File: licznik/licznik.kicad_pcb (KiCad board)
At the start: 2 copper layers, 72 x 44.1 mm, 66 parts, among them J4 1140084168, J5 Conn_01x03_Female, U1 AMS1117-3.3, U2 AMS1117-5.0, U6 oled, Y1 Crystal

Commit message: wip
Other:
- net class Default removed

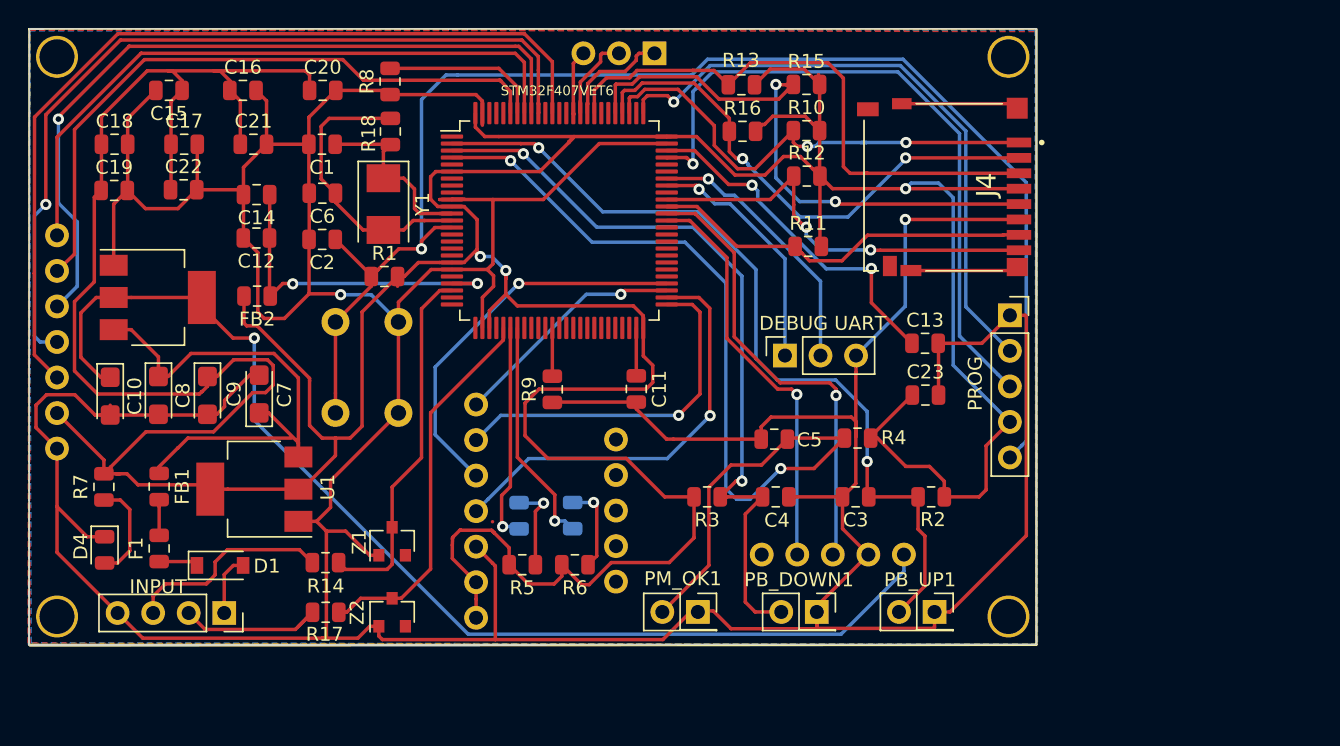
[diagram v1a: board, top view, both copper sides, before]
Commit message: hardware_2
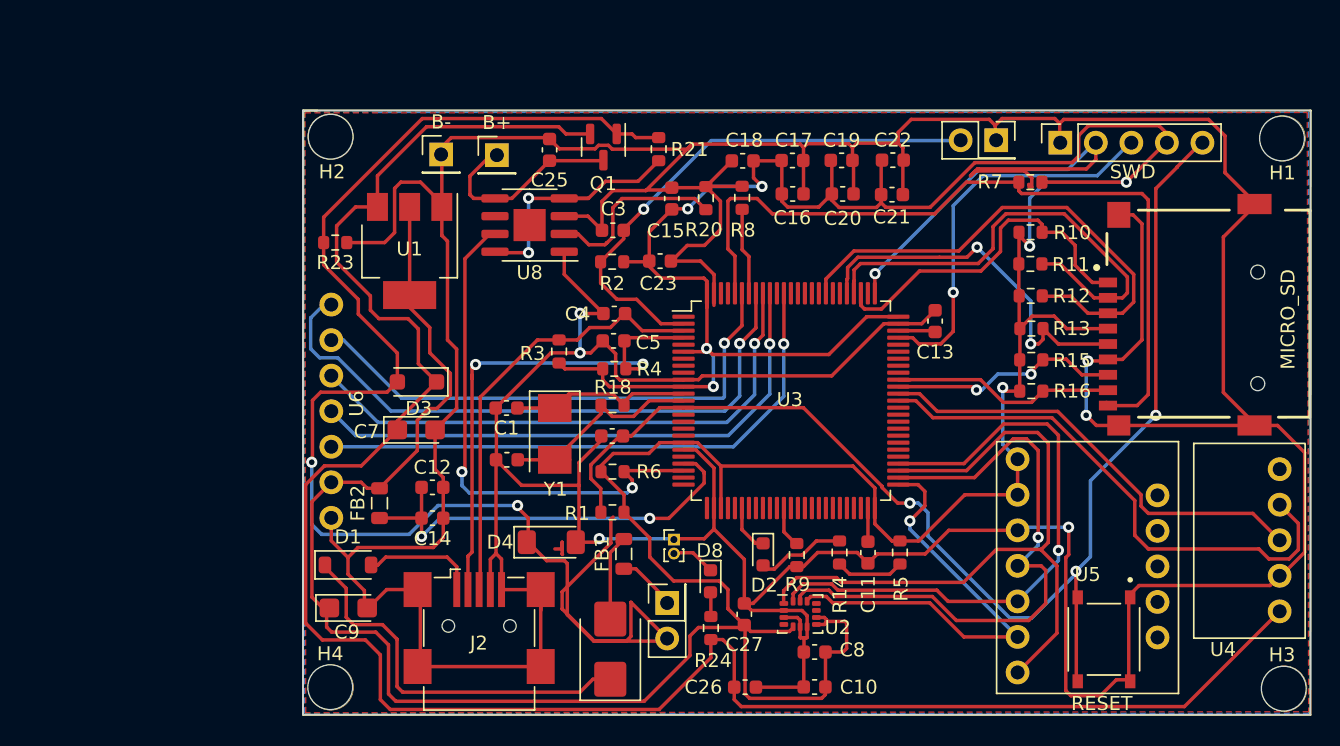
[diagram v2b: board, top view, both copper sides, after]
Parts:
- removed  LSM6DS3: gyro, licznik:gy1
- removed DEBUG UART: Conn_01x03_Female, Connector_PinSocket_2.54mm:PinSocket_1x03_P2.54mm_Vertical
- removed GPS NEO-6M: gps, licznik:gp1
- removed INPUT: Conn_01x04_Female, Connector_PinSocket_2.54mm:PinSocket_1x04_P2.54mm_Vertical
- removed J4: 1140084168, licznik:AMPHENOL_1140084168
- removed J5: Conn_01x03_Female, Connector_PinSocket_2.54mm:PinSocket_1x03_P2.54mm_Vertical
- removed PB_DOWN1, PB_UP1: SW_Push, Connector_PinSocket_2.54mm:PinSocket_2x01_P2.54mm_Vertical
- removed PM_OK1: PB_OK, Connector_PinSocket_2.54mm:PinSocket_2x01_P2.54mm_Vertical
- removed PROG: Conn_01x05_Female, Connector_PinSocket_2.54mm:PinSocket_1x05_P2.54mm_Vertical
- removed R17: 510R, Resistor_SMD:R_0805_2012Metric
- removed RESET1: SW_Push, Button_Switch_THT:SW_PUSH_6mm
- removed STM32F407VET6: STM32F407VETx, Package_QFP:LQFP-100_14x14mm_P0.5mm
- removed Z1, Z2: KDZ3.3V-RTK/P, Diode_SMD:D_SOT-23_ANK
- added B+: BAT+, Connector_PinHeader_2.54mm:PinHeader_1x01_P2.54mm_Vertical, F.Cu at (123.1, 71.7)
- added B-: BAT-, Connector_PinHeader_2.54mm:PinHeader_1x01_P2.54mm_Vertical, F.Cu at (119.1, 71.6)
- added C25: 10uF, Capacitor_SMD:C_0603_1608Metric, F.Cu at (126.8, 71.3)
- added C26: 22uF, Capacitor_SMD:C_0603_1608Metric, F.Cu at (140.8, 109.7)
- added C27: 22uF, Capacitor_SMD:C_0603_1608Metric, F.Cu at (140.8, 104.5)
- added D8: LED, LED_SMD:LED_0603_1608Metric, F.Cu at (138.4, 102.1)
- added H1: MountingHole_Pad, MountingHole:MountingHole_3.2mm_M3, F.Cu at (179.2, 70.5)
- added H2: MountingHole_Pad, MountingHole:MountingHole_3.2mm_M3, F.Cu at (111.2, 70.4)
- added H3: MountingHole_Pad, MountingHole:MountingHole_3.2mm_M3, F.Cu at (179.3, 109.8)
- added H4: MountingHole_Pad, MountingHole:MountingHole_3.2mm_M3, F.Cu at (111.2, 109.7)
- added J2: USB_B_Mini, Connector_USB:USB_Mini-B_Wuerth_65100516121_Horizontal, F.Cu at (121.8, 105.3)
- added LEN_ON: jump, Connector_PinHeader_1.00mm:PinHeader_1x02_P1.00mm_Vertical, F.Cu at (135.7, 99.2)
- added MICRO_SD: TF-01A, slot_sd:TF-01A, F.Cu at (173.9, 83.0)
- added PB_POWER: POWER_PB, Connector_PinSocket_2.54mm:PinSocket_2x01_P2.54mm_Vertical, F.Cu at (135.3, 103.7)
- added PB_UP: SW_Push, Connector_PinSocket_2.54mm:PinSocket_2x01_P2.54mm_Vertical, F.Cu at (158.8, 70.6)
- added Q1: AO3401A, Package_TO_SOT_SMD:SOT-23, F.Cu at (130.7, 71.1)
- added R20: 2K, Resistor_SMD:R_0603_1608Metric, F.Cu at (138.0, 74.8)
- added R21: 0.1R, Resistor_SMD:R_0603_1608Metric, F.Cu at (134.7, 71.2)
- added R23: 10K, Resistor_SMD:R_0603_1608Metric, F.Cu at (111.5, 77.9)
- added R24: 2K, Resistor_SMD:R_0603_1608Metric, F.Cu at (138.4, 105.5)
- added RESET: USER_PB, TS_1187A-B-A-B:SW_TS-1187A-B-A-B, F.Cu at (166.5, 106.3)
- added SWD: Conn_01x05_Female, Connector_PinSocket_2.54mm:PinSocket_1x05_P2.54mm_Vertical, F.Cu at (163.4, 70.8)
- added U3: STM32F407VETx, Package_QFP:LQFP-100_14x14mm_P0.5mm, F.Cu at (144.1, 89.2)
- added U4: gps, licznik:gp1, F.Cu at (176.7, 99.7)
- added U5: gyro, licznik:gy1, F.Cu at (165.3, 101.2)
- added U8: TP4056, Package_SO:HSOP-8-1EP_3.9x4.9mm_P1.27mm_EP2.3x2.3mm, F.Cu at (125.4, 76.7)
- C1, C11, C12, C13, C14, C15, C16, C17, C18, C19, C2, C20, C21, C22, C23, C3, C4, C5, C6: footprint Capacitor_SMD:C_0805_2012Metric -> Capacitor_SMD:C_0603_1608Metric
- C10, C8: value 10uF -> 100nF; footprint Capacitor_Tantalum_SMD:CP_EIA-3216-18_Kemet-A -> Capacitor_SMD:C_0603_1608Metric
- D2: footprint LED_SMD:LED_0805_2012Metric -> LED_SMD:LED_0603_1608Metric; moved to F.Cu
- D3: value LED -> SM4007; footprint LED_SMD:LED_0805_2012Metric -> Diode_SMD:D_SOD-123F; moved to F.Cu
- D4: value LED -> ZMMxx; footprint LED_SMD:LED_0805_2012Metric -> Diode_SMD:D_MiniMELF
- F1: footprint Fuse:Fuse_0805_2012Metric -> Diode_SMD:D_SMB
- R1, R10, R11, R12, R13, R15, R16, R18, R2, R3, R4, R5, R8, R9: footprint Resistor_SMD:R_0805_2012Metric -> Resistor_SMD:R_0603_1608Metric
- R14: value 510R -> 0R; footprint Resistor_SMD:R_0805_2012Metric -> Resistor_SMD:R_0603_1608Metric
- R6, R7: value 510R -> 10K; footprint Resistor_SMD:R_0805_2012Metric -> Resistor_SMD:R_0603_1608Metric
- U2: value AMS1117-5.0 -> LSM6DS3; footprint Package_TO_SOT_SMD:SOT-223-3_TabPin2 -> Package_LGA:LGA-14_3x2.5mm_P0.5mm_LayoutBorder3x4y
- moved R7 69.7 mm to (161.2, 73.6), turned to 0 degrees
- moved C10 54.5 mm to (145.8, 109.7), turned to 0 degrees
- moved C19 52.0 mm to (147.7, 72.0)
- moved U2 51.2 mm to (144.8, 104.5)
- moved C22 50.7 mm to (151.4, 72.0)
- moved C8 50.4 mm to (145.8, 107.2), turned to 180 degrees
- moved C21 45.8 mm to (151.3, 74.5)
- moved C18 44.9 mm to (140.7, 72.1), turned to 180 degrees
- moved C17 43.5 mm to (144.2, 72.1)
- moved C16 40.0 mm to (144.2, 74.5)
- moved C20 37.9 mm to (147.8, 74.5)
- moved C15 36.8 mm to (135.6, 74.8), turned to 90 degrees
- moved R14 36.7 mm to (147.6, 100.1), turned to -90 degrees
- moved FB1 33.6 mm to (132.2, 100.2), turned to 90 degrees
- moved F1 33.0 mm to (131.2, 107.0)
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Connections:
- C10 pad 1: +5V -> GND
- C10 pad 2: GND -> +3V3
- C7 pad 1: Net-(C7-Pad1) -> REG_IN
- C8 pad 1: Net-(C7-Pad1) -> +3V3
- D1 pad 2: +12V -> Net-(D1-A)
- D2 pad 2: Net-(D2-Pad2) -> Net-(D2-A)
- D3 pad 1: LED_2 -> REG_IN
- D3 pad 2: Net-(D3-Pad2) -> +5V
- D4 pad 1: GND -> +5V
- D4 pad 2: Net-(D4-Pad2) -> GND
- FB1 pad 1: Net-(C7-Pad1) -> Net-(FB1-Pad1)
- R11 pad 1: SDIO_D0 -> SDIO_D3
- R12 pad 1: SDIO_D1 -> SDIO_CMD
- R13 pad 1: SDIO_CMD -> SDIO_SCK
- R14 pad 1: Net-(J3-Pad3) -> Net-(D2-A)
- R14 pad 2: ENGINE_RPM_INPUT -> Net-(R14-Pad2)
- R15 pad 1: SDIO_SCK -> SDIO_D0
- R16 pad 1: SDIO_D3 -> SDIO_D1
- R5 pad 1: Net-(D2-Pad2) -> Net-(R14-Pad2)
- R6 pad 1: Net-(D3-Pad2) -> CHRG_SIGNAL
- R7 pad 1: Net-(D4-Pad2) -> SDIO_INSERT_CARD
- U1 pad 3: Net-(C7-Pad1) -> REG_IN
- U2 pad 1: GND -> GYRO_MISO
- U2 pad 2: +5V -> GND
- U2 pad 3: Net-(C7-Pad1) -> GND
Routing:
- net REG_IN: track 0.00 -> 145.0 mm
- net GND: track 373.0 -> 443.6 mm, vias 2 -> 6
- net SDIO_INSERT_CARD: track 0.00 -> 56.5 mm
- net +3V3: track 356.6 -> 308.7 mm, vias 3 -> 7
- net Net-(C7-Pad1): track 38.0 -> 0.00 mm
- net CHRG_SIGNAL: track 0.00 -> 37.4 mm, vias 0 -> 2
- net GYRO_MISO: track 17.0 -> 51.4 mm, vias 1 -> 0
- net PB_OK: track 70.1 -> 36.3 mm
- net +5V: track 82.0 -> 111.1 mm, vias 1 -> 2
- net WHEEL_RPM_INPUT: track 27.7 -> 0.00 mm
- net ENGINE_RPM_INPUT: track 26.0 -> 0.00 mm
- net Net-(D1-K): track 2.81 -> 27.9 mm
- net PB_DOWN: track 55.0 -> 31.3 mm, vias 2 -> 0
- net Net-(U3-VCAP_2): track 25.1 -> 2.97 mm, vias 2 -> 0
- net OLED_SCK: track 63.3 -> 41.2 mm, vias 0 -> 1
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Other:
- board size 72 x 44.1 mm -> 72 x 43.2 mm
- board text added: "GPS"
- board text added: "Gnd"
- board text added: "Rx"
- board text added: "Tx"
- board text added: "Vcc"
- board text removed: "12V"
- board text removed: "GND"
- board text removed: "Grzegorz W Licznik Motocyklowy"
- board text removed: "rpm"
- board text removed: "speed"

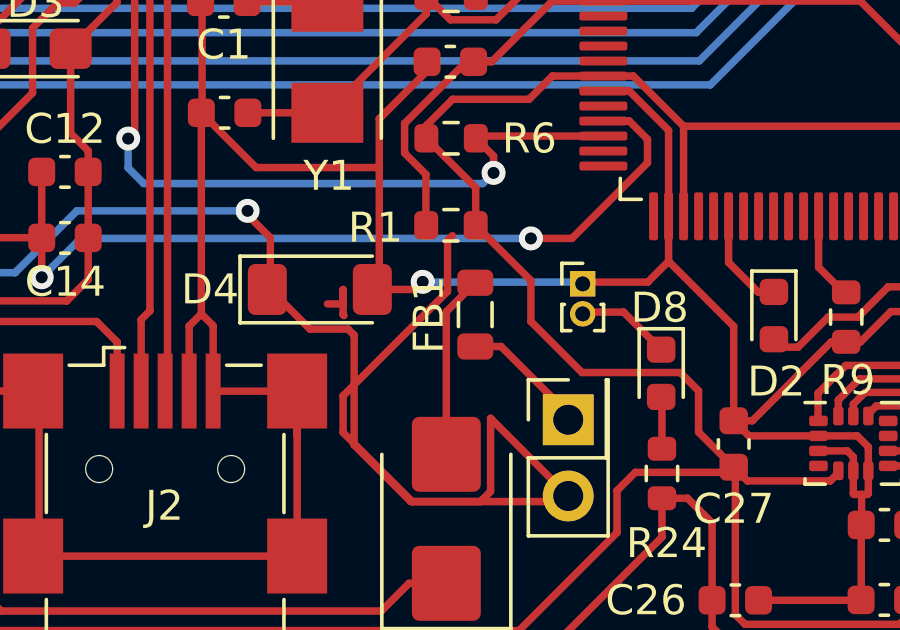
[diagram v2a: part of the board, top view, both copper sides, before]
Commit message: ulepszony pcb
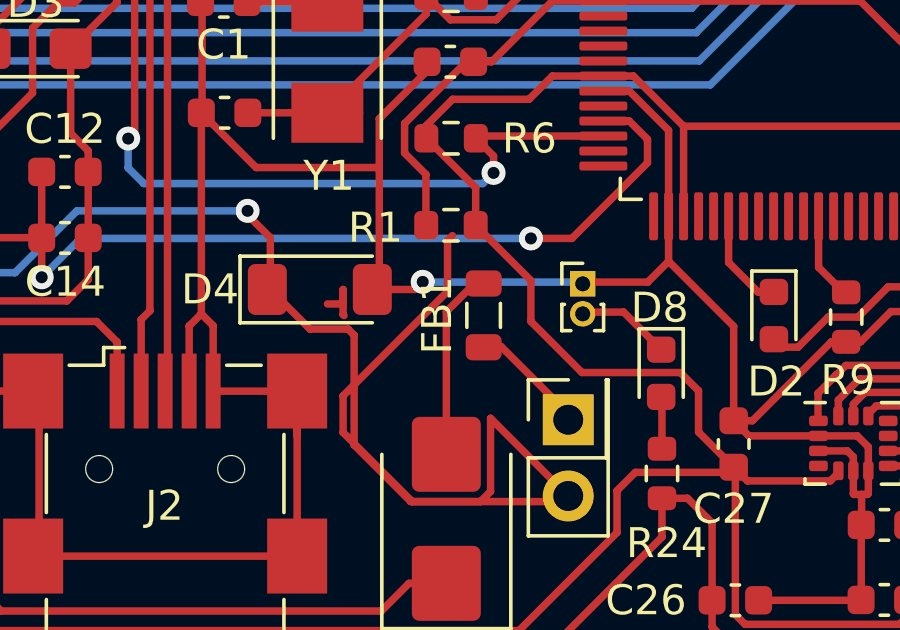
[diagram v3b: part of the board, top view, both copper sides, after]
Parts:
- moved FB1 0.28 mm to (132.4, 100.2)
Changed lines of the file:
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@@
   )
   (footprint "Inductor_SMD:L_0805_2012Metric" (layer "F.Cu")
-    (at 132.1562 100.1776 90)
+    (at 132.4356 100.203 90)
     (descr "Inductor SMD 0805 (2012 Metric), square (rectangular) end terminal, IPC_7351 nominal, (Body size source: IPC-SM-782 page 80, https://www.pcb-3d.com/wordpress/wp-content/uploads/ipc-sm-782a_amendment_1_and_2.pdf), generated with kicad-footprint-generator")
     (tags "inductor")
